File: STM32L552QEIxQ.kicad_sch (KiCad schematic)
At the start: 31 parts, among them U1 STM32L552QEIxQ, U2 TL431DBZ, Y1 ABM8G-24.000MHZ-4Y-T, Y2 ABS06-32.768KHZ-1-T

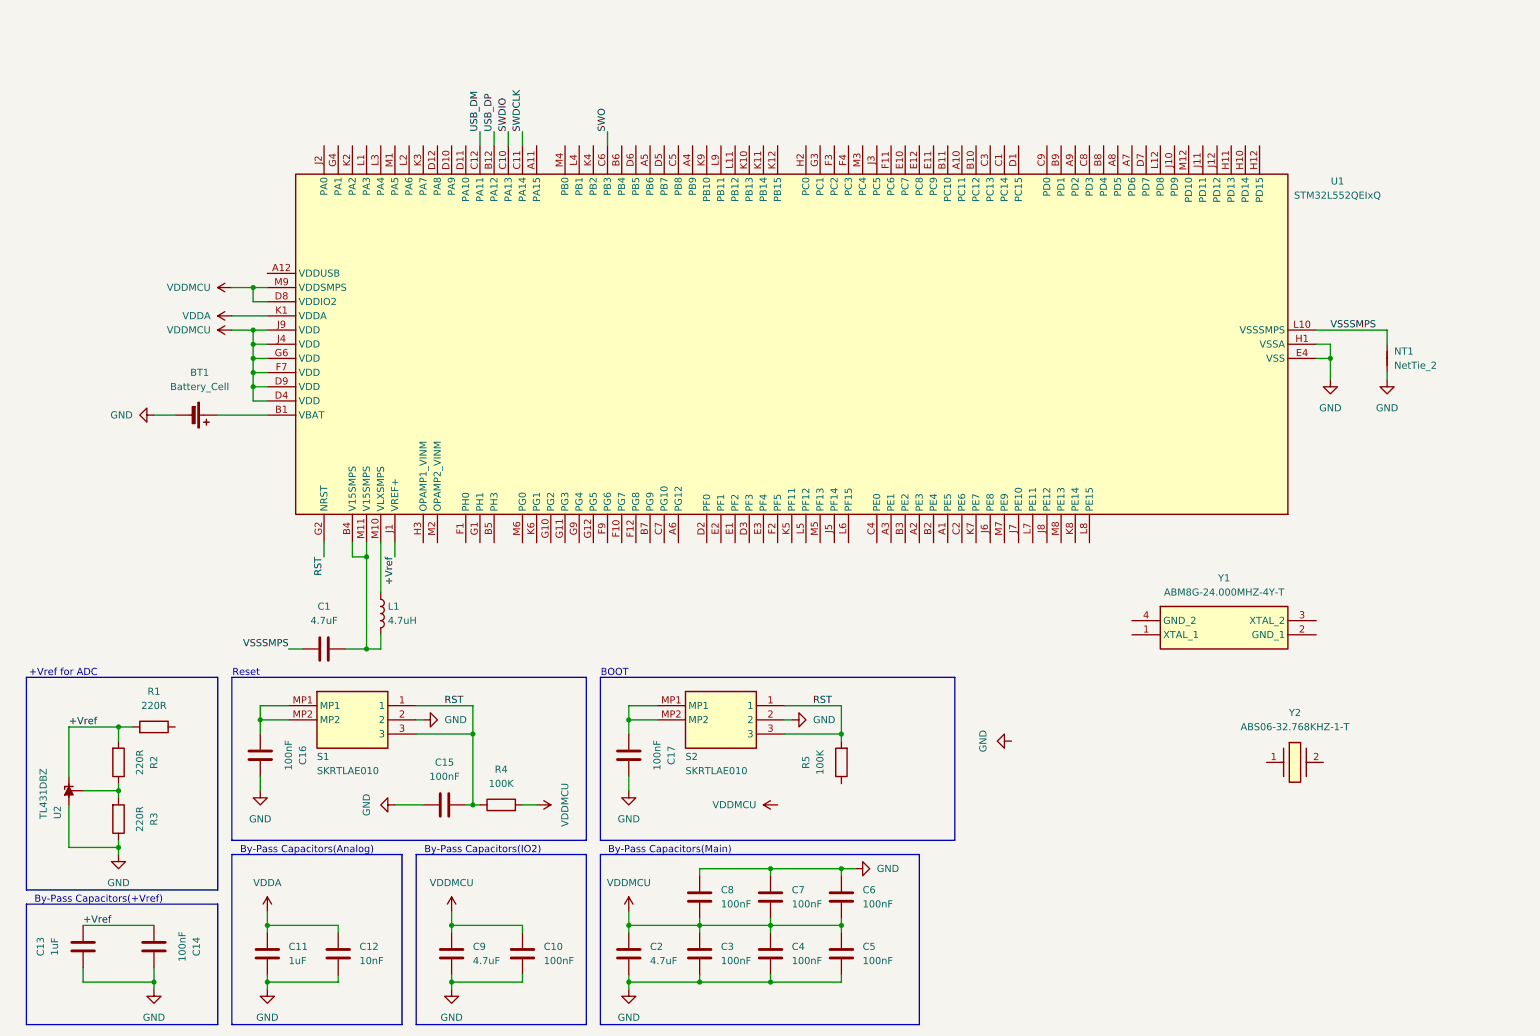
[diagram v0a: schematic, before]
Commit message: Commit_1
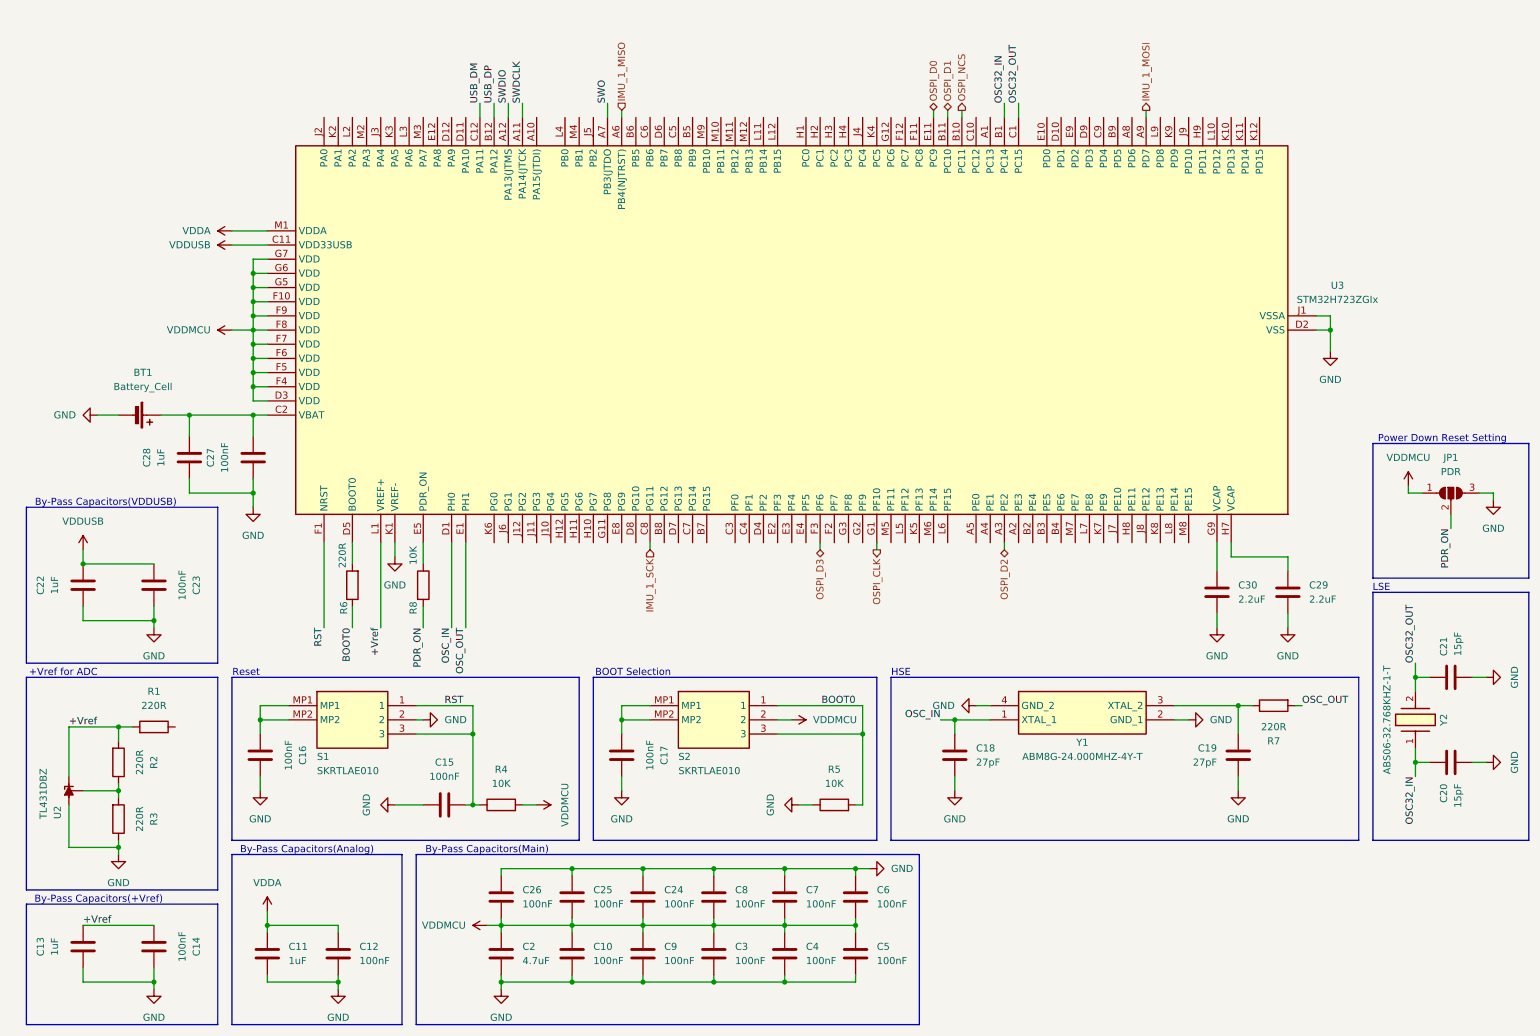
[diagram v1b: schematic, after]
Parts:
- removed C1: 4.7uF, Capacitor_SMD:C_0805_2012Metric, symbol Device:C
- removed L1: 4.7uH, Inductor_SMD:L_0805_2012Metric_Pad1.05x1.20mm_HandSolder, symbol Device:L
- removed NT1: NetTie_2, NetTie:NetTie-2_SMD_Pad0.5mm, symbol Device:NetTie_2
- removed U1: STM32L552QEIxQ, Package_BGA:UFBGA-132_7x7mm_Layout12x12_P0.5mm, symbol MCU_ST_STM32L5:STM32L552QEIxQ
- added C18, C19: 27pF, Capacitor_SMD:C_0805_2012Metric, symbol Device:C
- added C20, C21: 15pF, Capacitor_SMD:C_0805_2012Metric, symbol Device:C
- added C22, C28: 1uF, Capacitor_SMD:C_0805_2012Metric, symbol Device:C
- added C23, C24, C25, C26, C27: 100nF, Capacitor_SMD:C_0805_2012Metric, symbol Device:C
- added C29, C30: 2.2uF, Capacitor_SMD:C_0805_2012Metric, symbol Device:C
- added JP1: PDR, Jumper:SolderJumper-3_P2.0mm_Open_TrianglePad1.0x1.5mm_NumberLabels, symbol Jumper:SolderJumper_3_Open
- added R6, R7: 220R, Resistor_SMD:R_0805_2012Metric, symbol Device:R
- added R8: 10K, Resistor_SMD:R_0805_2012Metric, symbol Device:R
- added U3: STM32H723ZGIx, Package_BGA:UFBGA-144_7x7mm_Layout12x12_P0.5mm, symbol MCU_ST_STM32H7:STM32H723ZGIx
- C12: value 10nF -> 100nF
- C9: value 4.7uF -> 100nF
- R4, R5: value 100K -> 10K
- Y2: footprint ABS06 -> ABS06:ABS06
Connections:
- net +Vref: now also U3.L1 (VREF+)
- net GND: now also R5.1, Y1.2 (GND_1), Y1.4 (GND_2), C18.2, C19.2, C20.2, C21.2, C22.1, C23.1, C24.1, C25.1, C26.1, C27.2, C28.1, C29.1, C30.1, JP1.3 (B), U3.D2 (VSS), U3.E6 (VSS), U3.E7 (VSS), U3.G10 (VSS), U3.G4 (VSS), U3.G8 (VSS), U3.H5 (VSS), U3.H6 (VSS), U3.J1 (VSSA), U3.K1 (VREF-); no longer S2.2
- net RST: now also U3.F1 (NRST); no longer R5.2, S2.1, S2.3
- net SWDCLK: now also U3.A11 (PA14(JTCK)
- net SWDIO: now also U3.A12 (PA13(JTMS)
- net SWO: now also U3.A7 (PB3(JTDO)
- net USB_DM: now also U3.C12 (PA11)
- net USB_DP: now also U3.B12 (PA12)
- net VDDA: now also U3.M1 (VDDA)
- net VDDMCU: now also S2.2, C24.2, C25.2, C26.2, JP1.1 (A), U3.D3 (VDD), U3.F10 (VDD), U3.F4 (VDD), U3.F5 (VDD), U3.F6 (VDD), U3.F7 (VDD), U3.F8 (VDD), U3.F9 (VDD), U3.G5 (VDD), U3.G6 (VDD), U3.G7 (VDD)
- net OSC32_IN: now reaches Y2.1
- net OSC32_IN: now also C20.1, U3.B1 (PC14)
- net OSC32_OUT: now reaches Y2.2
- net OSC32_OUT: now also C21.1, U3.C1 (PC15)
- net OSC_IN: now reaches Y1.1 (XTAL_1)
- net OSC_IN: now also C18.1, U3.D1 (PH0)
- net at Y1.3 (XTAL_2): now also C19.1, R7.1
- net at BT1.1 (+): now also C27.1, C28.2, U3.C2 (VBAT)
- new net: R6.2, U3.D5 (BOOT0)
- new net: R8.1, U3.E5 (PDR_ON)
- new net: C30.2, U3.G9 (VCAP)
- new net: C29.2, U3.H7 (VCAP)
- new net BOOT0: R5.2, R6.1, S2.1, S2.3
- new net IMU_1_MISO: U3.A6 (PB4(NJTRST))
- new net IMU_1_MOSI: U3.A9 (PD7)
- new net IMU_1_SCK: U3.C8 (PG11)
- new net OSC_OUT: R7.2, U3.E1 (PH1)
- new net OSPI_CLK: U3.G1 (PF10)
- new net OSPI_D0: U3.E11 (PC9)
- new net OSPI_D1: U3.B11 (PC10)
- new net OSPI_D2: U3.A3 (PE2)
- new net OSPI_D3: U3.F3 (PF6)
- new net OSPI_NCS: U3.B10 (PC11)
- new net PDR_ON: JP1.2 (C), R8.2
- new net VDDUSB: C22.2, C23.2, U3.C11 (VDD33USB)
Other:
- note added: "BOOT Selection"
- note added: "By-Pass Capacitors(VDDUSB)"
- note added: "HSE"
- note added: "LSE"
- note added: "Power Down Reset Setting"
- note removed: "BOOT"
- note removed: "By-Pass Capacitors(IO2)"
- moved on the sheet: BT1, C10, C17, C2, C3, C4, C5, C6, C7, C8, C9, R5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

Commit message: progress
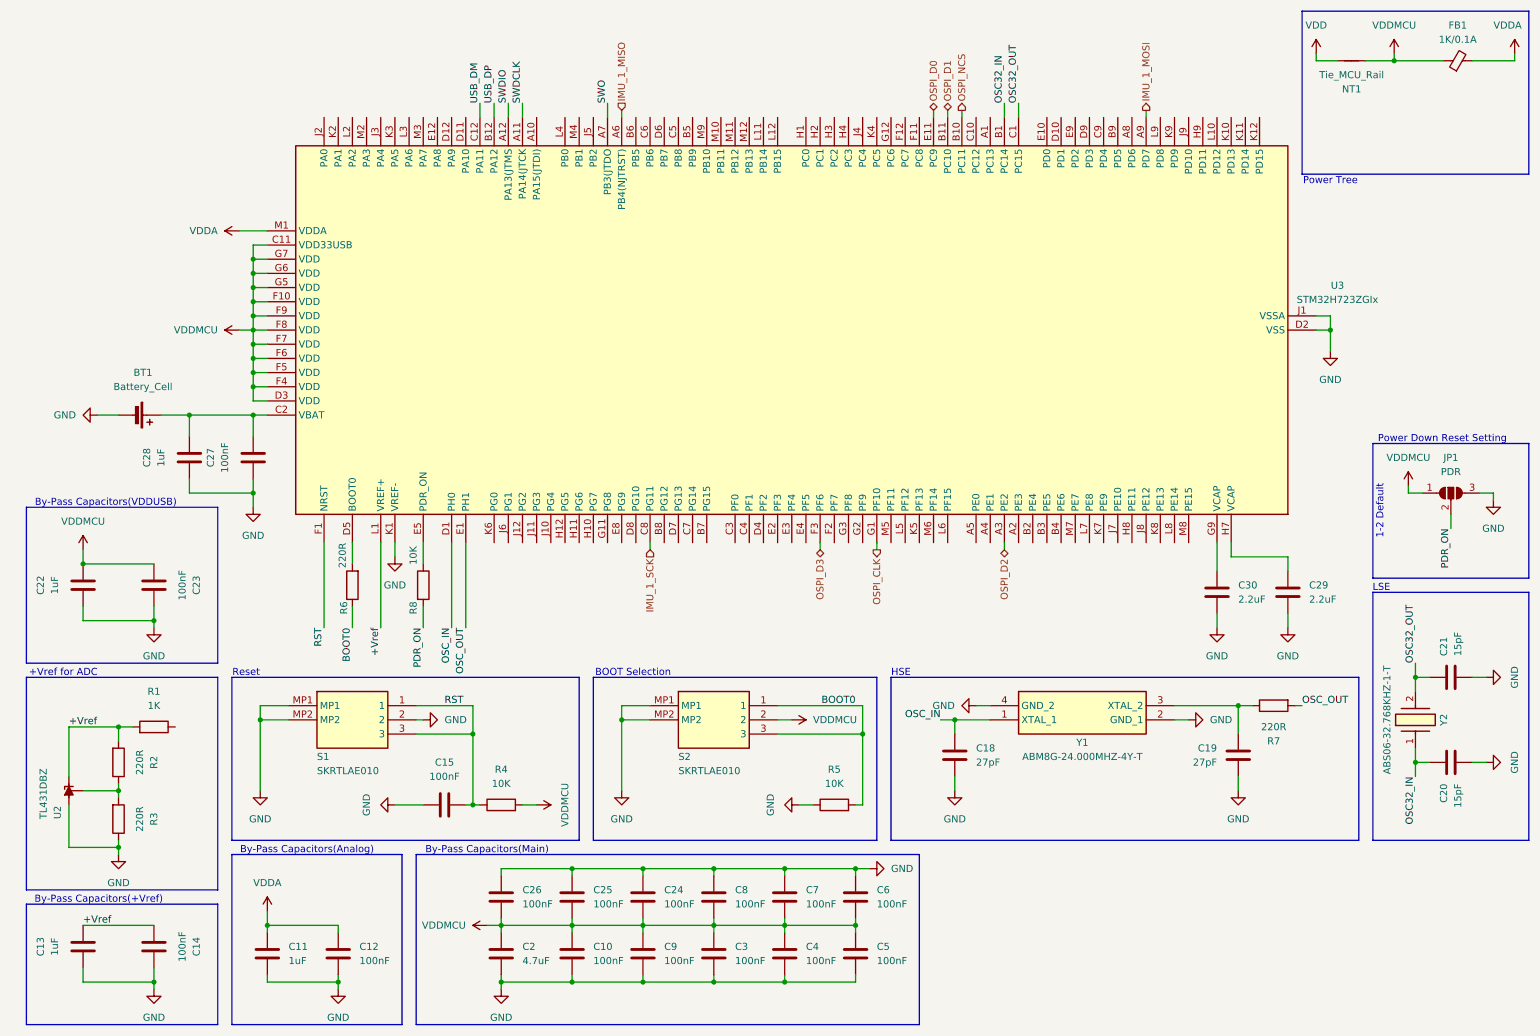
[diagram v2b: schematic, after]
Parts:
- removed C16, C17: 100nF, Capacitor_SMD:C_0805_2012Metric, symbol Device:C
- added FB1: 1K/0.1A, Inductor_SMD:L_0603_1608Metric, symbol Device:FerriteBead_Small
- added NT1: Tie_MCU_Rail, NetTie:NetTie-2_SMD_Pad0.5mm, symbol Device:NetTie_2
- R1: value 220R -> 1K
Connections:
- net VDDUSB is gone; now on net VDDMCU: C22.2, C23.2, U3.C11 (VDD33USB)
- net GND: now also S1.MP1, S1.MP2, S2.MP1, S2.MP2
- net VDDA: now also FB1.2
- net VDDMCU: now also FB1.1, NT1.2
- new net VDD: NT1.1
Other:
- note added: "1-2 Default"
- note added: "Power Tree"
